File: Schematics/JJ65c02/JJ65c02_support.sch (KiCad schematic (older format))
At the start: 29 parts, among them SW1 RESET, U1 NE555, U2 74HC00, U3 74AC138, U4 74HC08, U5 MAX232B, U6 LM386, X1 1Mhz, X2 1.8Mhz

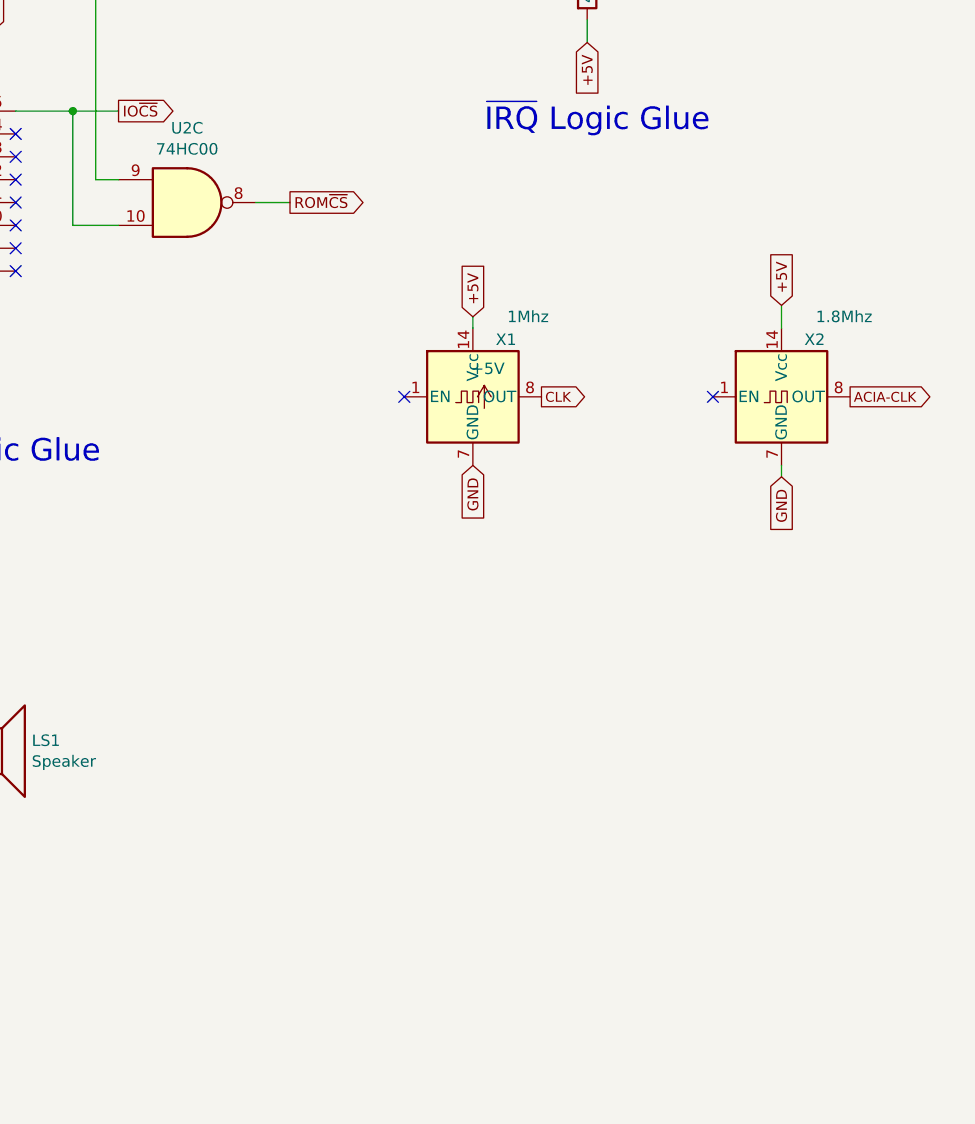
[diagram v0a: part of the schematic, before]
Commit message: 2nd VIA
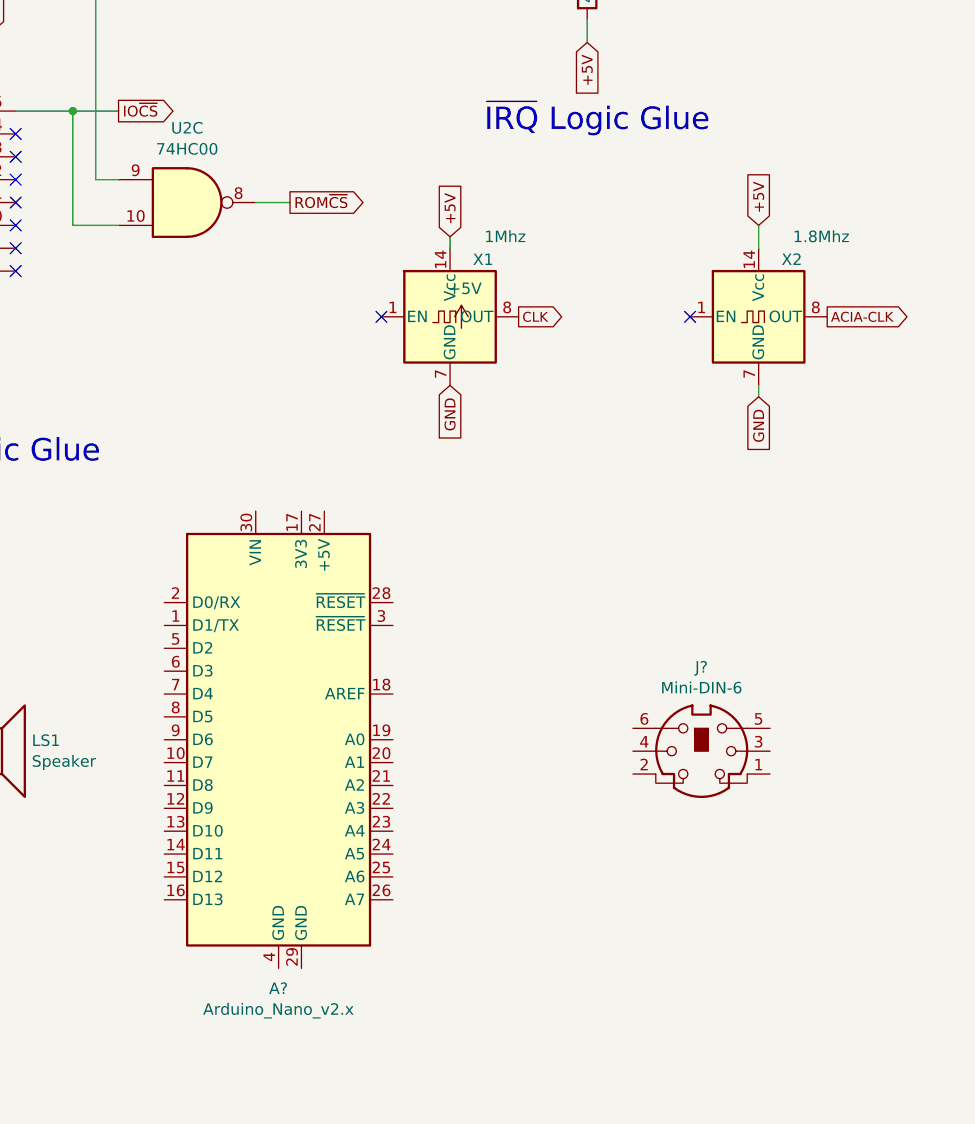
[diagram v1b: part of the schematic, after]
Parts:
- added A?: Arduino_Nano_v2.x, Module:Arduino_Nano, symbol MCU_Module:Arduino_Nano_v2.x
- added J?: Mini-DIN-6, symbol Connector:Mini-DIN-6
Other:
- moved on the sheet: X1, X2
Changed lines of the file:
@@
 L Oscillator:CXO_DIP14 X?
 U 1 1 6171CEB1
-P 8800 3650
+P 8700 3300
 AR Path="/6171CEB1" Ref="X?"  Part="1"
 AR Path="/61660CAC/6171CEB1" Ref="X1"  Part="1"
 AR Path="/61610474/6171CEB1" Ref="X?"  Part="1"
-F 0 "X1" H 8900 3900 50  0000 L CNN
-F 1 "1Mhz" H 8950 4000 50  0000 L CNN
-F 2 "Oscillator:Oscillator_DIP-14" H 9250 3300 50  0001 C CNN
-F 3 "http://cdn-reichelt.de/documents/datenblatt/B400/OSZI.pdf" H 8700 3650 50  0001 C CNN
-	1    8800 3650
-	1    0    0    -1
-$EndComp
-Text GLabel 9100 3650 2    43   Output ~ 0
+F 0 "X1" H 8800 3550 50  0000 L CNN
+F 1 "1Mhz" H 8850 3650 50  0000 L CNN
+F 2 "Oscillator:Oscillator_DIP-14" H 9150 2950 50  0001 C CNN
+F 3 "http://cdn-reichelt.de/documents/datenblatt/B400/OSZI.pdf" H 8600 3300 50  0001 C CNN
+	1    8700 3300
+	1    0    0    -1
+$EndComp
+Text GLabel 9000 3300 2    43   Output ~ 0
 CLK
 $Comp
 L power:+5V #PWR?
 U 1 1 6171CEBE
-P 8850 3700
+P 8750 3350
 AR Path="/6171CEBE" Ref="#PWR?"  Part="1"
 AR Path="/61660CAC/6171CEBE" Ref="#PWR020"  Part="1"
 AR Path="/61610474/6171CEBE" Ref="#PWR?"  Part="1"
-F 0 "#PWR020" H 8850 3550 50  0001 C CNN
-F 1 "+5V" H 8865 3873 50  0000 C CNN
-F 2 "" H 8850 3700 50  0001 C CNN
-F 3 "" H 8850 3700 50  0001 C CNN
-	1    8850 3700
-	1    0    0    -1
-$EndComp
-NoConn ~ 8500 3650
+F 0 "#PWR020" H 8750 3200 50  0001 C CNN
+F 1 "+5V" H 8765 3523 50  0000 C CNN
+F 2 "" H 8750 3350 50  0001 C CNN
+F 3 "" H 8750 3350 50  0001 C CNN
+	1    8750 3350
+	1    0    0    -1
+$EndComp
+NoConn ~ 8400 3300
 $Comp
 L Oscillator:CXO_DIP14 X?
 U 1 1 6171CEC5
-P 10150 3650
+P 10050 3300
 AR Path="/6171CEC5" Ref="X?"  Part="1"
 AR Path="/61660CAC/6171CEC5" Ref="X2"  Part="1"
 AR Path="/61610474/6171CEC5" Ref="X?"  Part="1"
-F 0 "X2" H 10250 3900 50  0000 L CNN
-F 1 "1.8Mhz" H 10300 4000 50  0000 L CNN
-F 2 "Oscillator:Oscillator_DIP-14" H 10600 3300 50  0001 C CNN
-F 3 "http://cdn-reichelt.de/documents/datenblatt/B400/OSZI.pdf" H 10050 3650 50  0001 C CNN
-	1    10150 3650
-	1    0    0    -1
-$EndComp
-Text GLabel 10450 3650 2    43   Output ~ 0
+F 0 "X2" H 10150 3550 50  0000 L CNN
+F 1 "1.8Mhz" H 10200 3650 50  0000 L CNN
+F 2 "Oscillator:Oscillator_DIP-14" H 10500 2950 50  0001 C CNN
+F 3 "http://cdn-reichelt.de/documents/datenblatt/B400/OSZI.pdf" H 9950 3300 50  0001 C CNN
+	1    10050 3300
+	1    0    0    -1
+$EndComp
+Text GLabel 10350 3300 2    43   Output ~ 0
 ACIA-CLK
-NoConn ~ 9850 3650
+NoConn ~ 9750 3300
 $Comp
 L 74xx:74HC00 U2
@@
 a12
 Wire Wire Line
-	8800 3300 8800 3350
+	8700 2950 8700 3000
 $Comp
 L 74xx:74LS138 U3
@@
 Text GLabel 1200 2400 0    47   Input ~ 0
 GND
-Text GLabel 10150 4000 3    47   Input ~ 0
+Text GLabel 10050 3650 3    47   Input ~ 0
 GND
 Text GLabel 6300 3500 3    47   Input ~ 0
@@
 Text GLabel 6700 2050 1    47   Input ~ 0
 +5V
-Text GLabel 8800 3300 1    47   Input ~ 0
-+5V
-Text GLabel 10150 3250 1    47   Input ~ 0
-+5V
-Text GLabel 8800 3950 3    47   Input ~ 0
-GND
-Wire Wire Line
-	10150 3250 10150 3350
-Wire Wire Line
-	10150 3950 10150 4000
+Text GLabel 8700 2950 1    47   Input ~ 0
++5V
+Text GLabel 10050 2900 1    47   Input ~ 0
++5V
+Text GLabel 8700 3600 3    47   Input ~ 0
+GND
+Wire Wire Line
+	10050 2900 10050 3000
+Wire Wire Line
+	10050 3600 10050 3650
 $Comp
 L 74xx:74LS08 U4
@@
 Wire Wire Line
 	4450 6350 4200 6350
+$Comp
+L MCU_Module:Arduino_Nano_v2.x A?
+U 1 1 61B02721
+P 7950 5150
+F 0 "A?" H 7950 4061 50  0000 C CNN
+F 1 "Arduino_Nano_v2.x" H 7950 3970 50  0000 C CNN
+F 2 "Module:Arduino_Nano" H 7950 5150 50  0001 C CIN
+F 3 "https://www.arduino.cc/en/uploads/Main/ArduinoNanoManual23.pdf" H 7950 5150 50  0001 C CNN
+	1    7950 5150
+	1    0    0    -1
+$EndComp
+$Comp
+L Connector:Mini-DIN-6 J?
+U 1 1 61B062BD
+P 9800 5200
+F 0 "J?" H 9800 5567 50  0000 C CNN
+F 1 "Mini-DIN-6" H 9800 5476 50  0000 C CNN
+F 2 "" H 9800 5200 50  0001 C CNN
+F 3 "http://service.powerdynamics.com/ec/Catalog17/Section%2011.pdf" H 9800 5200 50  0001 C CNN
+	1    9800 5200
+	1    0    0    -1
+$EndComp
 Wire Bus Line
 	1000 6400 1000 6500
